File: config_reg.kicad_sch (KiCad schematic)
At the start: 1 part, among them U9 74HC273

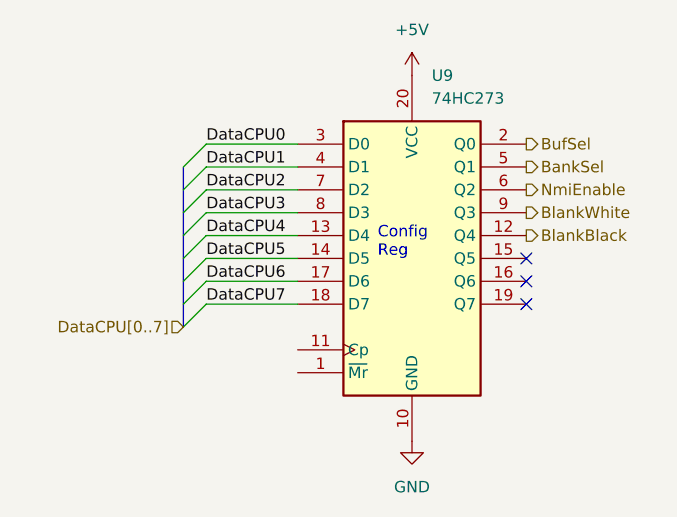
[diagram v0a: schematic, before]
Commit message: work on DAC
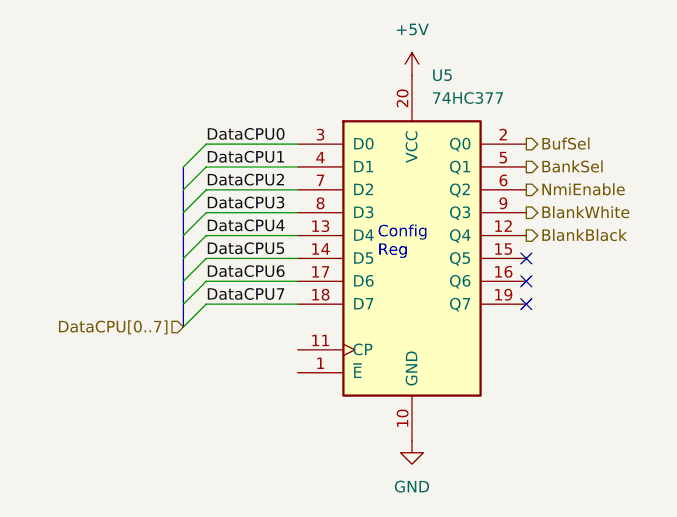
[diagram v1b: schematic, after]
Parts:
- removed U9: 74HC273, symbol 74xx:74HC273
- added U5: 74HC377, symbol 74xx:74LS377
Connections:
- net +5V: now also U5.20 (VCC)
- net BankSel: now also U5.5 (Q1)
- net BlankBlack: now also U5.12 (Q4)
- net BlankWhite: now also U5.9 (Q3)
- net BufSel: now also U5.2 (Q0)
- net DataCPU0: now also U5.3 (D0)
- net DataCPU1: now also U5.4 (D1)
- net DataCPU2: now also U5.7 (D2)
- net DataCPU3: now also U5.8 (D3)
- net DataCPU4: now also U5.13 (D4)
- net DataCPU5: now also U5.14 (D5)
- net DataCPU6: now also U5.17 (D6)
- net DataCPU7: now also U5.18 (D7)
- net GND: now also U5.10 (GND)
- net NmiEnable: now also U5.6 (Q2)
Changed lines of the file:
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@@
+    )
+  )
+  (symbol (lib_id "74xx:74LS377") (at 124.46 97.79 0) (unit 1)
+    (in_bom yes) (on_board yes) (dnp no) (fields_autoplaced)
+    (property "Reference" "U5" (at 126.6541 77.47 0)
+      (effects (font (size 1.27 1.27)) (justify left))
+    )
+    (property "Value" "74HC377" (at 126.6541 80.01 0)
+      (effects (font (size 1.27 1.27)) (justify left))
+    )
+    (property "Footprint" "" (at 124.46 97.79 0)
+      (effects (font (size 1.27 1.27)) hide)
+    )
+    (property "Datasheet" "http://www.ti.com/lit/gpn/sn74LS377" (at 124.46 97.79 0)
+      (effects (font (size 1.27 1.27)) hide)
+    )
+    (pin "1")
+    (pin "10")
+    (pin "11")
+    (pin "12")
+    (pin "13")
+    (pin "14")
+    (pin "15")
+    (pin "16")
+    (pin "17")
+    (pin "18")
+    (pin "19")
+    (pin "2")
+    (pin "20")
+    (pin "3")
+    (pin "4")
+    (pin "5")
+    (pin "6")
+    (pin "7")
+    (pin "8")
+    (pin "9")
+    (instances
+      (project "6502gpu"
+        (path "/b1d8dca2-c863-4452-b293-53802be895cc/25d51073-b007-4d3a-a895-244d96d772f9"
+          (reference "U5") (unit 1)
+        )
+      )
     )
   )
@@
         )
       )
-    )
-  )
-  (symbol (lib_id "74xx:74HC273") (at 124.46 97.79 0) (unit 1)
-    (in_bom yes) (on_board yes) (dnp no)
-    (property "Reference" "U9" (at 126.6541 77.47 0)
-      (effects (font (size 1.27 1.27)) (justify left))
-    )
-    (property "Value" "74HC273" (at 126.6541 80.01 0)
-      (effects (font (size 1.27 1.27)) (justify left))
-    )
-    (property "Footprint" "" (at 124.46 97.79 0)
-      (effects (font (size 1.27 1.27)) hide)
-    )
-    (property "Datasheet" "https://assets.nexperia.com/documents/data-sheet/74HC_HCT273.pdf" (at 124.46 97.79 0)
-      (effects (font (size 1.27 1.27)) hide)
-    )
-    (pin "1")
-    (pin "10")
-    (pin "11")
-    (pin "12")
-    (pin "13")
-    (pin "14")
-    (pin "15")
-    (pin "16")
-    (pin "17")
-    (pin "18")
-    (pin "19")
-    (pin "2")
-    (pin "20")
-    (pin "3")
-    (pin "4")
-    (pin "5")
-    (pin "6")
-    (pin "7")
-    (pin "8")
-    (pin "9")
-    (instances
-      (project "6502gpu"
-        (path "/b1d8dca2-c863-4452-b293-53802be895cc/25d51073-b007-4d3a-a895-244d96d772f9"
-          (reference "U9") (unit 1)
-        )
-      )

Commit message: work on main page layout
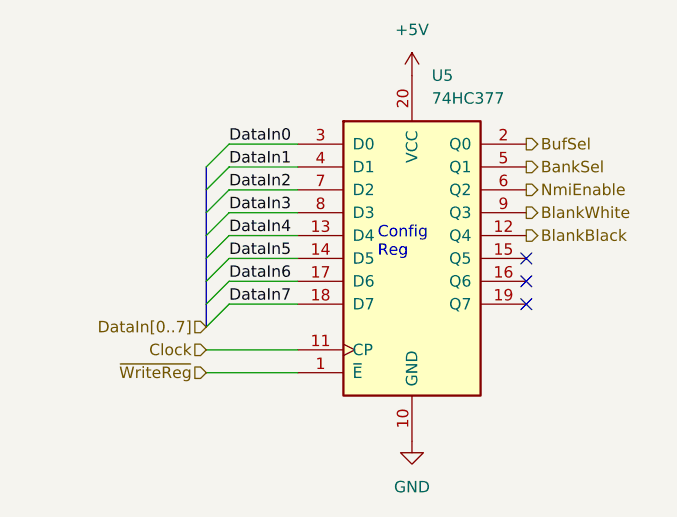
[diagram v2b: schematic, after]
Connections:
- net ~{WriteReg}: now reaches U5.1 (~{E})
- net Clock: now reaches U5.11 (CP)
- net DataCPU0 renamed DataIn0
- net DataCPU1 renamed DataIn1
- net DataCPU2 renamed DataIn2
- net DataCPU3 renamed DataIn3
- net DataCPU4 renamed DataIn4
- net DataCPU5 renamed DataIn5
- net DataCPU6 renamed DataIn6
- net DataCPU7 renamed DataIn7
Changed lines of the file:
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@@
   (no_connect (at 137.16 100.33))
   (no_connect (at 137.16 102.87))
-  (bus_entry (at 101.6 100.33) (size -2.54 2.54)
+  (bus_entry (at 104.14 100.33) (size -2.54 2.54)
     (stroke (width 0) (type default))
   )
-  (bus_entry (at 101.6 87.63) (size -2.54 2.54)
+  (bus_entry (at 104.14 87.63) (size -2.54 2.54)
     (stroke (width 0) (type default))
   )
-  (bus_entry (at 101.6 92.71) (size -2.54 2.54)
+  (bus_entry (at 104.14 92.71) (size -2.54 2.54)
     (stroke (width 0) (type default))
   )
-  (bus_entry (at 101.6 102.87) (size -2.54 2.54)
+  (bus_entry (at 104.14 102.87) (size -2.54 2.54)
     (stroke (width 0) (type default))
   )
-  (bus_entry (at 101.6 90.17) (size -2.54 2.54)
+  (bus_entry (at 104.14 90.17) (size -2.54 2.54)
     (stroke (width 0) (type default))
   )
-  (bus_entry (at 101.6 97.79) (size -2.54 2.54)
+  (bus_entry (at 104.14 97.79) (size -2.54 2.54)
     (stroke (width 0) (type default))
   )
-  (bus_entry (at 101.6 95.25) (size -2.54 2.54)
+  (bus_entry (at 104.14 95.25) (size -2.54 2.54)
     (stroke (width 0) (type default))
   )
-  (bus_entry (at 101.6 85.09) (size -2.54 2.54)
+  (bus_entry (at 104.14 85.09) (size -2.54 2.54)
     (stroke (width 0) (type default))
   )
-  (bus (pts (xy 99.06 102.87) (xy 99.06 105.41))
+  (wire (pts (xy 101.6 107.95) (xy 111.76 107.95))
     (stroke (width 0) (type default))
   )
-  (wire (pts (xy 111.76 97.79) (xy 101.6 97.79))
+  (bus (pts (xy 101.6 102.87) (xy 101.6 105.41))
     (stroke (width 0) (type default))
   )
-  (bus (pts (xy 99.06 100.33) (xy 99.06 102.87))
+  (wire (pts (xy 111.76 97.79) (xy 104.14 97.79))
     (stroke (width 0) (type default))
   )
-  (wire (pts (xy 111.76 92.71) (xy 101.6 92.71))
+  (bus (pts (xy 101.6 100.33) (xy 101.6 102.87))
     (stroke (width 0) (type default))
   )
-  (wire (pts (xy 111.76 102.87) (xy 101.6 102.87))
+  (wire (pts (xy 101.6 110.49) (xy 111.76 110.49))
     (stroke (width 0) (type default))
   )
-  (bus (pts (xy 99.06 90.17) (xy 99.06 92.71))
+  (wire (pts (xy 111.76 92.71) (xy 104.14 92.71))
     (stroke (width 0) (type default))
   )
-  (wire (pts (xy 111.76 90.17) (xy 101.6 90.17))
+  (wire (pts (xy 111.76 102.87) (xy 104.14 102.87))
     (stroke (width 0) (type default))
   )
-  (bus (pts (xy 99.06 95.25) (xy 99.06 97.79))
+  (bus (pts (xy 101.6 90.17) (xy 101.6 92.71))
     (stroke (width 0) (type default))
   )
-  (bus (pts (xy 99.06 92.71) (xy 99.06 95.25))
+  (wire (pts (xy 111.76 90.17) (xy 104.14 90.17))
     (stroke (width 0) (type default))
   )
-  (bus (pts (xy 99.06 87.63) (xy 99.06 90.17))
+  (bus (pts (xy 101.6 95.25) (xy 101.6 97.79))
     (stroke (width 0) (type default))
   )
-  (wire (pts (xy 111.76 95.25) (xy 101.6 95.25))
+  (bus (pts (xy 101.6 92.71) (xy 101.6 95.25))
     (stroke (width 0) (type default))
   )
-  (wire (pts (xy 111.76 87.63) (xy 101.6 87.63))
+  (bus (pts (xy 101.6 87.63) (xy 101.6 90.17))
     (stroke (width 0) (type default))
   )
-  (wire (pts (xy 111.76 100.33) (xy 101.6 100.33))
+  (wire (pts (xy 111.76 95.25) (xy 104.14 95.25))
     (stroke (width 0) (type default))
   )
-  (bus (pts (xy 99.06 97.79) (xy 99.06 100.33))
+  (wire (pts (xy 111.76 87.63) (xy 104.14 87.63))
     (stroke (width 0) (type default))
   )
-  (wire (pts (xy 111.76 85.09) (xy 101.6 85.09))
+  (wire (pts (xy 111.76 100.33) (xy 104.14 100.33))
+    (stroke (width 0) (type default))
+  )
+  (bus (pts (xy 101.6 97.79) (xy 101.6 100.33))
+    (stroke (width 0) (type default))
+  )
+  (wire (pts (xy 111.76 85.09) (xy 104.14 85.09))
     (stroke (width 0) (type default))
   )
@@
     (effects (font (size 1.27 1.27)) (justify left bottom))
   )
-  (label "DataCPU1" (at 101.6 87.63 0) (fields_autoplaced)
+  (label "DataIn1" (at 104.14 87.63 0) (fields_autoplaced)
     (effects (font (size 1.27 1.27)) (justify left bottom))
   )
-  (label "DataCPU0" (at 101.6 85.09 0) (fields_autoplaced)
+  (label "DataIn0" (at 104.14 85.09 0) (fields_autoplaced)
     (effects (font (size 1.27 1.27)) (justify left bottom))
   )
-  (label "DataCPU6" (at 101.6 100.33 0) (fields_autoplaced)
+  (label "DataIn6" (at 104.14 100.33 0) (fields_autoplaced)
     (effects (font (size 1.27 1.27)) (justify left bottom))
   )
-  (label "DataCPU4" (at 101.6 95.25 0) (fields_autoplaced)
+  (label "DataIn4" (at 104.14 95.25 0) (fields_autoplaced)
     (effects (font (size 1.27 1.27)) (justify left bottom))
   )
-  (label "DataCPU2" (at 101.6 90.17 0) (fields_autoplaced)
+  (label "DataIn2" (at 104.14 90.17 0) (fields_autoplaced)
     (effects (font (size 1.27 1.27)) (justify left bottom))
   )
-  (label "DataCPU5" (at 101.6 97.79 0) (fields_autoplaced)
+  (label "DataIn5" (at 104.14 97.79 0) (fields_autoplaced)
     (effects (font (size 1.27 1.27)) (justify left bottom))
   )
-  (label "DataCPU7" (at 101.6 102.87 0) (fields_autoplaced)
+  (label "DataIn7" (at 104.14 102.87 0) (fields_autoplaced)
     (effects (font (size 1.27 1.27)) (justify left bottom))
   )
-  (label "DataCPU3" (at 101.6 92.71 0) (fields_autoplaced)
+  (label "DataIn3" (at 104.14 92.71 0) (fields_autoplaced)
     (effects (font (size 1.27 1.27)) (justify left bottom))
   )
-  (hierarchical_label "DataCPU[0..7]" (shape input) (at 99.06 105.41 180) (fields_autoplaced)
+  (hierarchical_label "~{WriteReg}" (shape input) (at 101.6 110.49 180) (fields_autoplaced)
+    (effects (font (size 1.27 1.27)) (justify right))
+  )
+  (hierarchical_label "DataIn[0..7]" (shape input) (at 101.6 105.41 180) (fields_autoplaced)
     (effects (font (size 1.27 1.27)) (justify right))
   )
@@
     (effects (font (size 1.27 1.27)) (justify left))
   )
+  (hierarchical_label "Clock" (shape input) (at 101.6 107.95 180) (fields_autoplaced)
+    (effects (font (size 1.27 1.27)) (justify right))
+  )
   (hierarchical_label "BankSel" (shape output) (at 137.16 87.63 0) (fields_autoplaced)
